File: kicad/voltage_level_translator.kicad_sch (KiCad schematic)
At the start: 16 parts, among them Q1 2N7002, Q2 2N7002, Q3 2N7002, U4 LSF0108PW, U5 LSF0108PW, U6 LSF0108PW

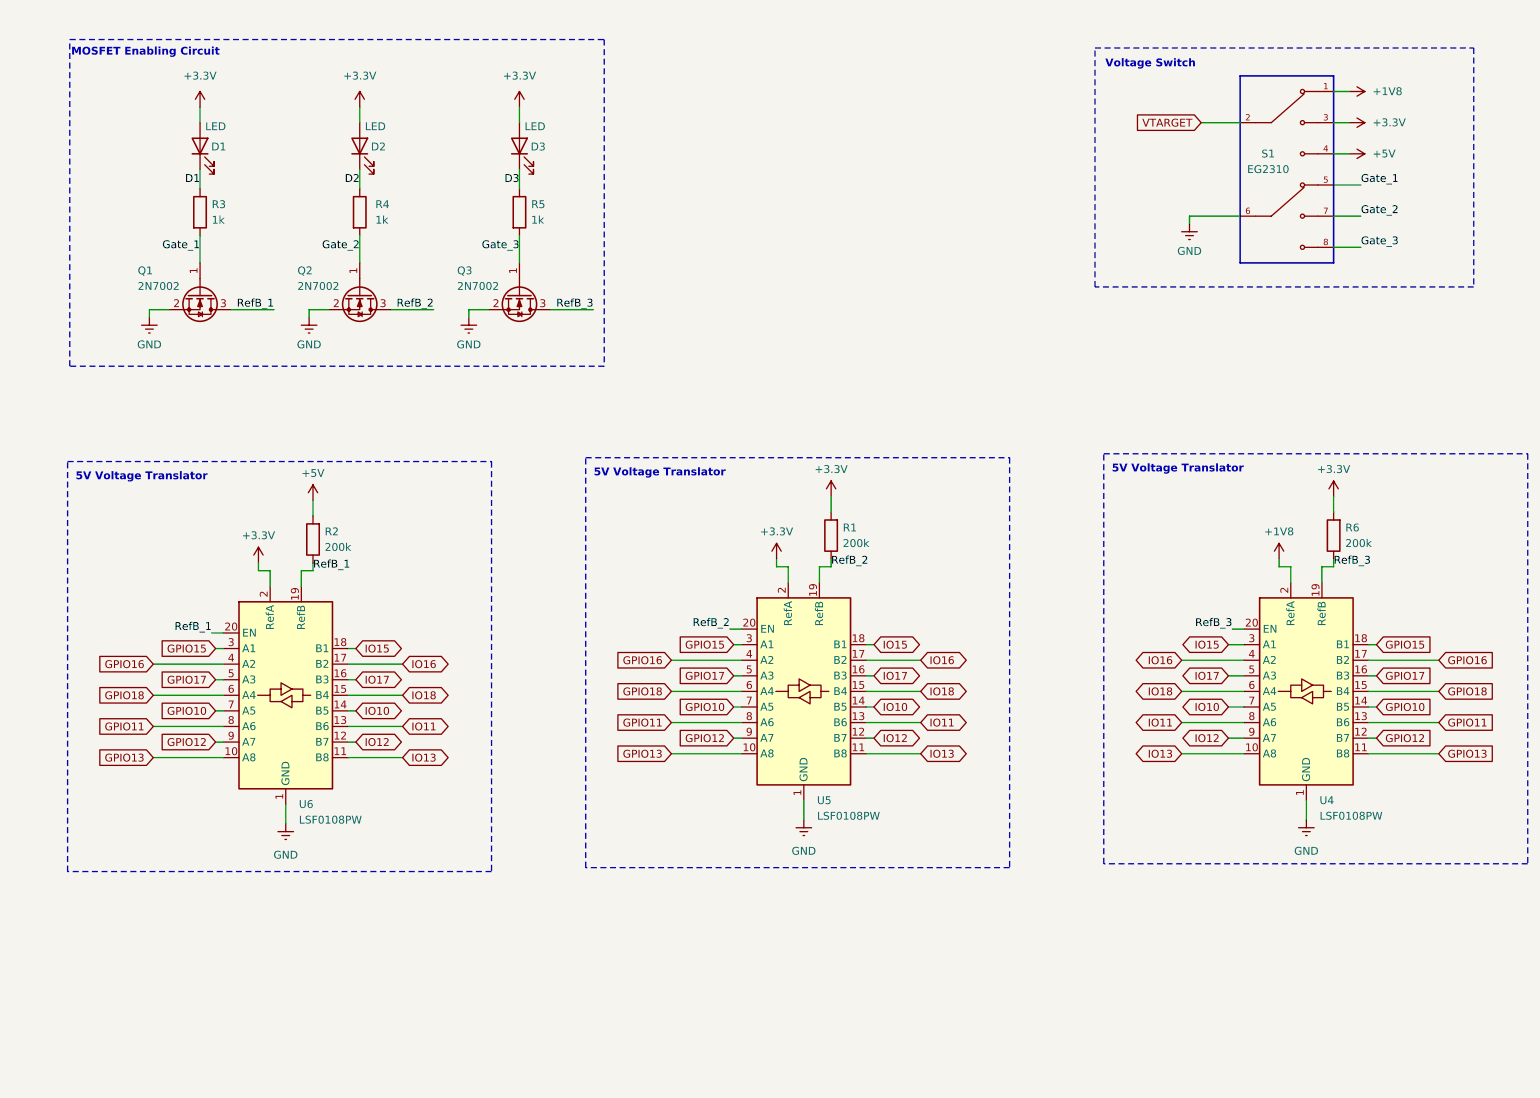
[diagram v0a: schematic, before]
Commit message: Experimented with wiring
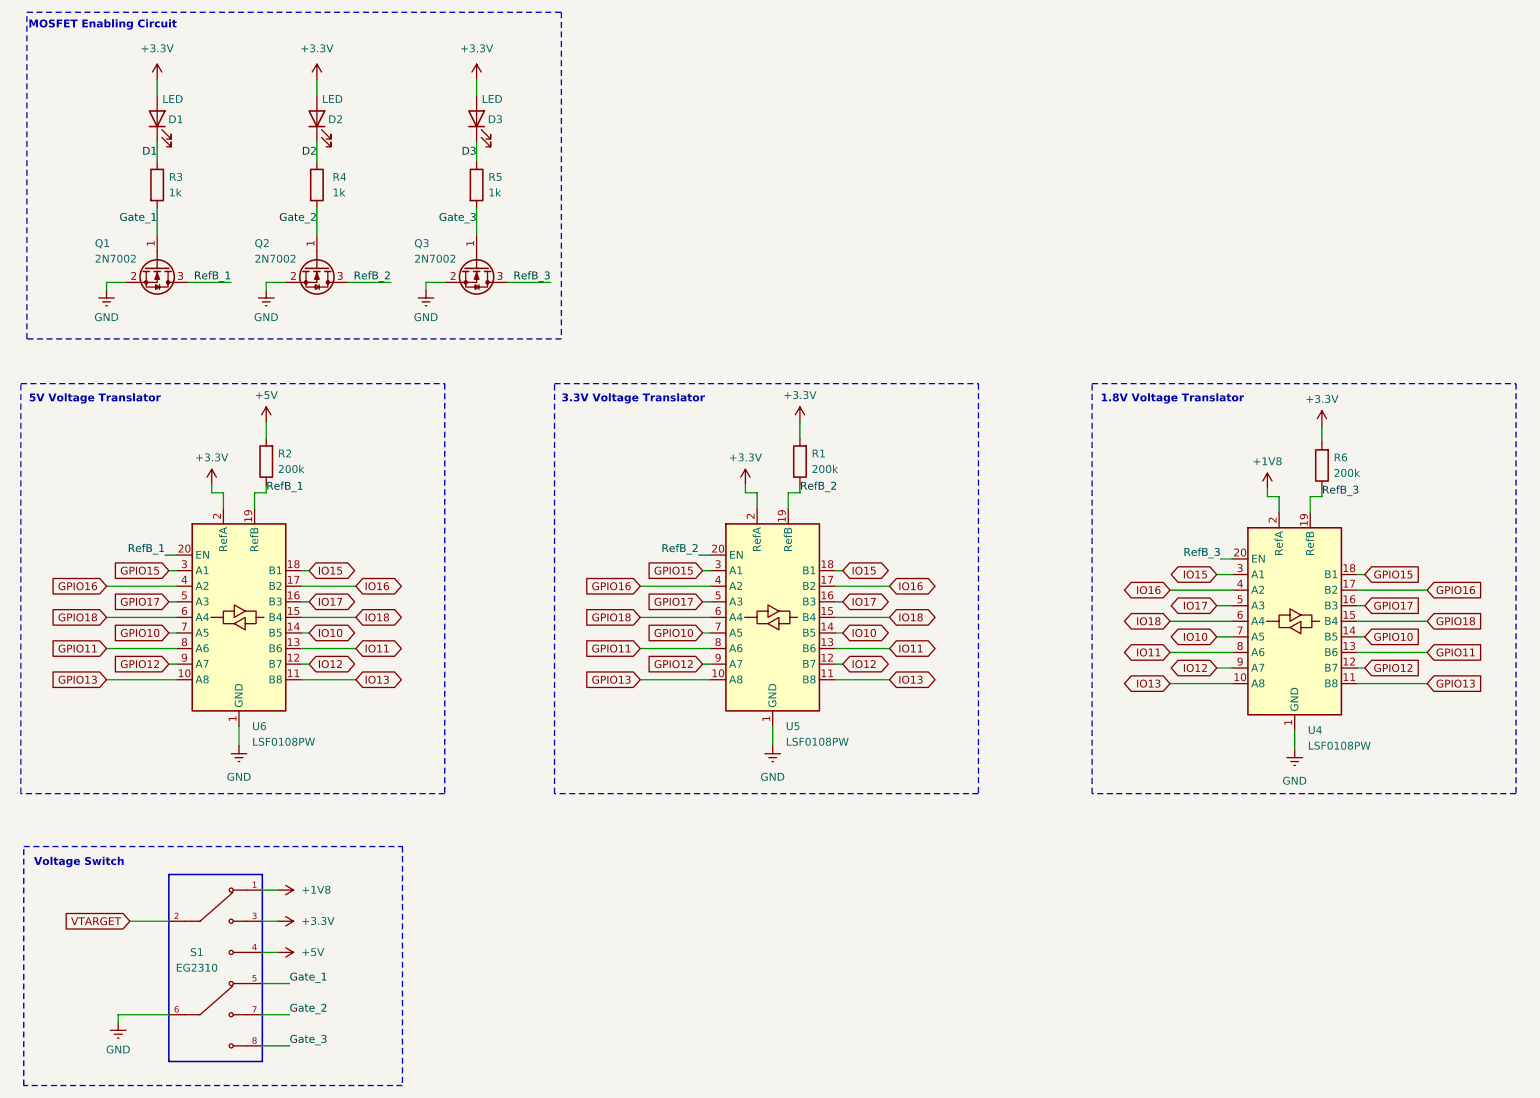
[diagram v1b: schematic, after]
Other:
- note added: "1.8V Voltage Translator"
- note added: "3.3V Voltage Translator"
- moved on the sheet: D1, D2, D3, Q1, Q2, Q3, R1, R2, R3, R4, R5, R6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

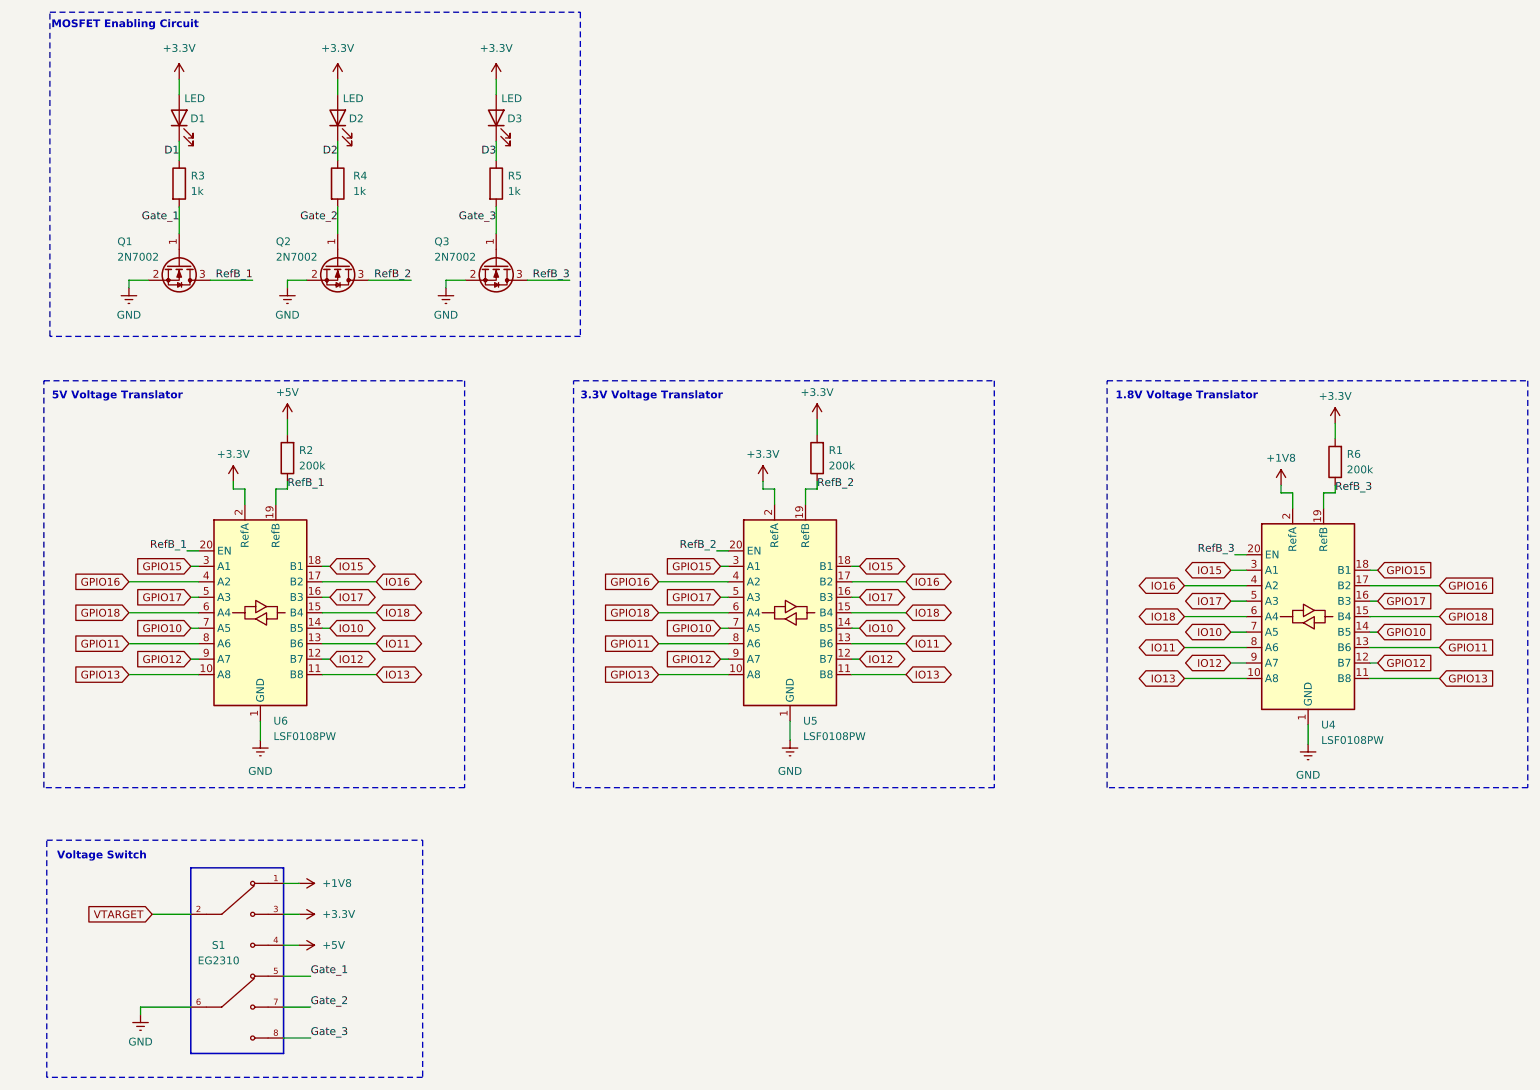
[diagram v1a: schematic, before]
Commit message: Updated PCB
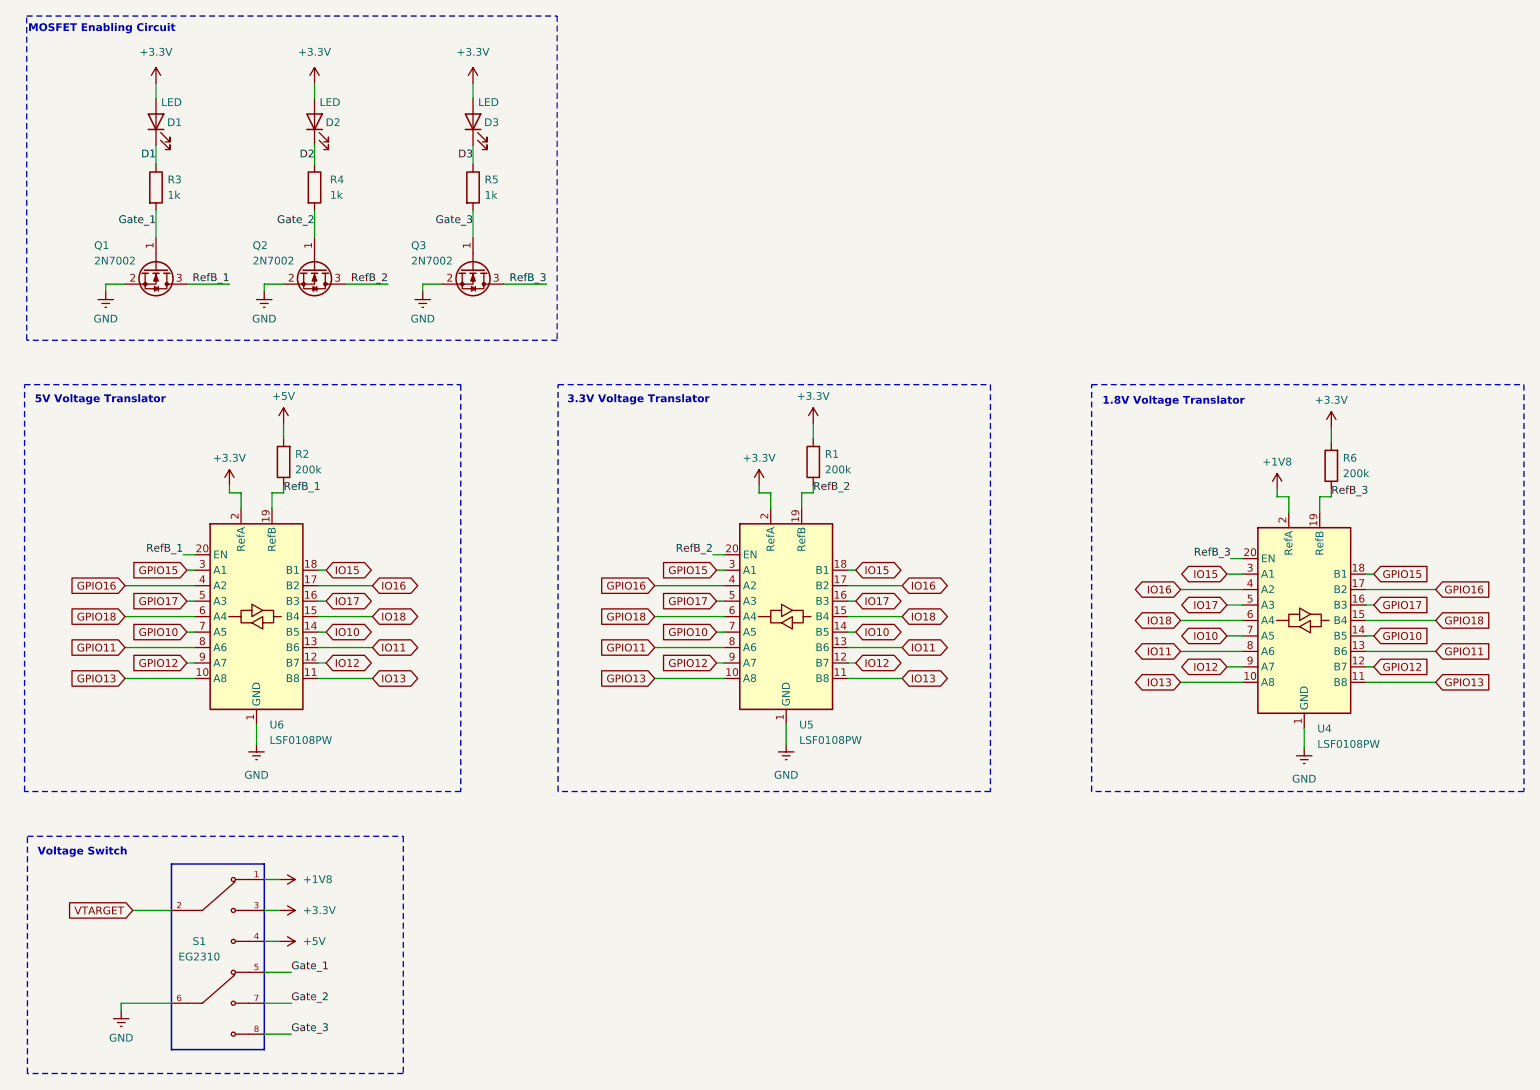
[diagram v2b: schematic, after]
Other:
- moved on the sheet: D1, D2, D3, Q1, Q2, Q3, R1, R2, R3, R4, R5, R6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

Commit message: Update voltage_level_translator.kicad_sch
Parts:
- added U3, U7: TMUX1574PW, Package_SO:TSSOP-16_4.4x5mm_P0.65mm, symbol Analog_Switch:TMUX1574PW
- added U8, U9: TXS0108EPW, Package_SO:Texas_PW0020A_TSSOP-20_4.4x6.5mm_P0.65mm, symbol Logic_LevelTranslator:TXS0108EPW
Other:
- moved on the sheet: D1, D2, D3, Q1, Q2, Q3, R1, R2, R3, R4, R5, R6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
